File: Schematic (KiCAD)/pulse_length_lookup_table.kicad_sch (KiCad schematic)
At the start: 122 parts

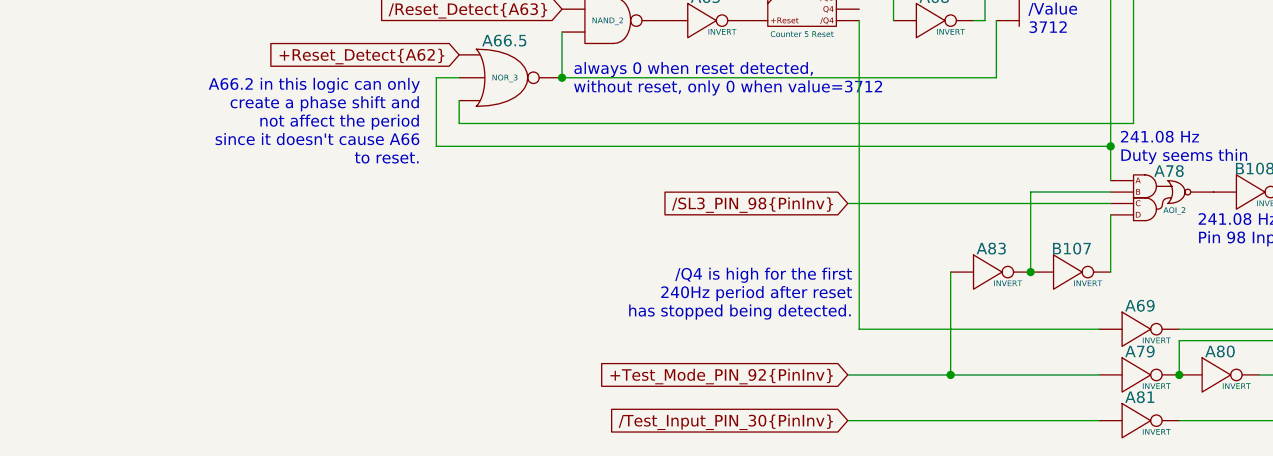
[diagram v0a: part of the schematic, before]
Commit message: Schematic and SVG Updates
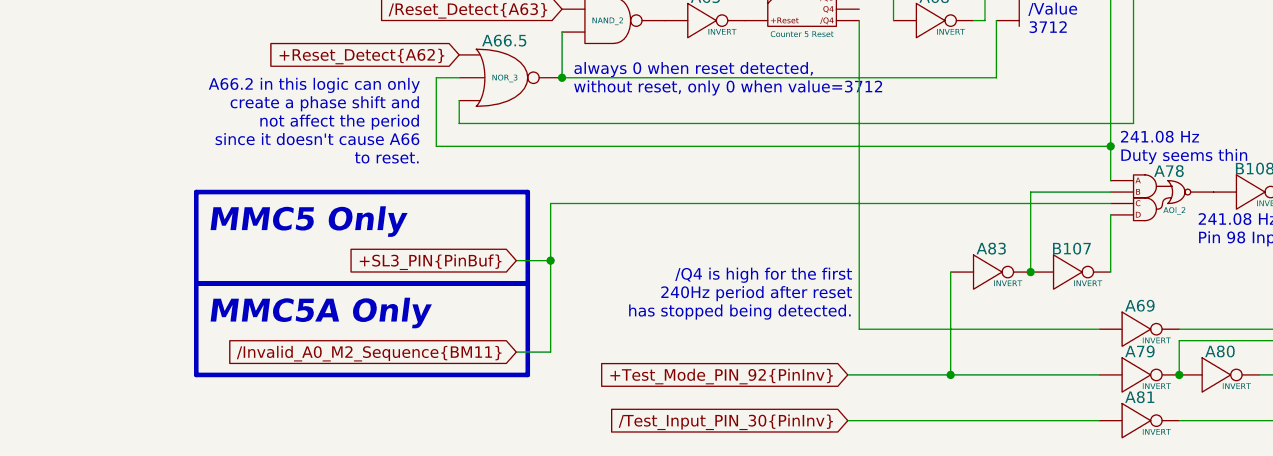
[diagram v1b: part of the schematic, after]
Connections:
- net /SL3_PIN_98{PinInv} is gone; now on net +SL3_PIN{PinBuf}: A78. (X)
- net at B108. (X): now also A78. (X); no longer A70. (X)
- net at A71. (X): now also A72. (X), A73. (X); no longer A70. (X)
- net at C16. (X): now also D47. (X); no longer C15. (X)
- net at D45. (X): now also D46. (X); no longer C16. (X)
- net at D47. (X): now also D48. (X); no longer C16. (X)
- net at D72. (X): now also C22. (X); no longer D71. (X)
- net at D92. (X): now also C26. (X); no longer D91. (X)
- net at C26. (X): now also C25. (X); no longer D92. (X)
- net at C18. (X): now also D51. (X); no longer C17. (X)
- net at D106. (X): now also C28. (X); no longer D105. (X)
- net at A58. (X): now also A57. (X), A66. (/Q7); no longer A59. (X)
- net at D66. (X): now also D65. (X); no longer C20. (X)
- net at A67. (/Q4): now also A65. (X)
- net at A66.7. (X): now also A66.4. (X); no longer A67. (/Q4)
- net at A68. (X): now also A66.4. (X); no longer A67. (/Q4)
- net at A66.6. (X): now also A66.4. (X); no longer A67. (/Q4)
- net at A69. (X): now also A77. (X); no longer A67. (/Q4)
- net at A65. (X): now also A64. (X); no longer A67. (/Q4)
- net at A66.4. (X): now also A66.5. (X), A78. (X); no longer A66.7. (X)
- net at D64. (X): now also C20. (X); no longer D63. (X)
- net at D76. (X): now also C22. (X); no longer D75. (X)
- net at D53. (X): now also C18. (X); no longer D54. (X)
- net at D96. (X): now also D95. (X); no longer C26. (X)
- net at A73. (X): now also A74. (X); no longer A82. (X)
- net at A74. (X): now also A75. (X); no longer A73. (X)
- net at D49. (X): now also C18. (X); no longer D50. (X)
- net at D55. (X): now also C18. (X); no longer D56. (X)
- net at D74. (X): now also D73. (X); no longer C22. (X)
- net at D70. (X): now also D69. (X); no longer C22. (X)
- net at D68. (X): now also D67. (X); no longer C22. (X)
- net at A77. (X): now also A82. (X); no longer A81. (X)
- net at A77. (X), A80. (X): now also A79. (X)
- net at D104. (X): now also C28. (X); no longer D103. (X)
- net at C28. (X): now also C27. (X); no longer D104. (X)
- net at D58. (X): now also C20. (X); no longer D57. (X)
- net at C20. (X): now also D62. (X); no longer D58. (X)
- net at A66.3. (X): now also A66. (/Q7); no longer A66.4. (X)
- net at D78. (X): now also C24. (X); no longer D77. (X)
- net at C24. (X): now also D88. (X); no longer D78. (X)
- net at D102. (X): now also C28. (X); no longer D101. (X)
- net at D51. (X): now also D52. (X); no longer C18. (X)
- net at D100. (X): now also C26. (X); no longer D99. (X)
- net at D60. (X): now also C20. (X); no longer D59. (X)
- net at D84. (X): now also D83. (X); no longer C24. (X)
- net at D86. (X): now also C24. (X); no longer D85. (X)
- net +SL3_PIN{PinBuf}: now reaches A78. (X)
- net +SL3_PIN{PinBuf}: no longer B108. (X)
- net at D82. (X): now also D81. (X); no longer C24. (X)
- net at D80. (X): now also D79. (X); no longer C24. (X)
- net at D90. (X): now also C26. (X); no longer D89. (X)
- net at A60. (X): now also A56. (X); no longer A61. (X)
- net at D94. (X): now also C26. (X); no longer D93. (X)
- net at A66.2. (X): now also A66.5. (X); no longer A66. (/Q7)
- net at D98. (X): now also D97. (X); no longer C26. (X)
- new net: A70. (X), B108. (X)
- new net: A70. (X), A71. (X)
- new net: C15. (X), C16. (X)
- new net: C16. (X), D45. (X)
- new net: D71. (X), D72. (X)
- new net: D91. (X), D92. (X)
- new net: C17. (X), C18. (X)
- new net: D105. (X), D106. (X)
- new net: A58. (X), A59. (X)
- new net: C20. (X), D66. (X)
- new net: A66.7. (X), A67. (/Q4)
- new net: A67. (/Q4), A68. (X)
- new net: A66.6. (X), A67. (/Q4)
- new net: A67. (/Q4), A69. (X)
- new net: A66. (/Q7), A67. (/Q4)
- new net: D63. (X), D64. (X)
- new net: D75. (X), D76. (X)
- new net: D53. (X), D54. (X)
- new net: C26. (X), D96. (X)
- new net: A73. (X), A82. (X)
- new net: D49. (X), D50. (X)
- new net: A64. (X), A66.4. (X), A66.5. (X)
- new net: D55. (X), D56. (X)
- new net: C21. (X), C22. (X)
- new net: C22. (X), D74. (X)
- new net: C22. (X), D70. (X)
- new net: C22. (X), D68. (X)
- new net: A77. (X), A81. (X)
- new net: A77. (X), A80. (X)
- new net: D103. (X), D104. (X)
- new net: D57. (X), D58. (X)
- new net: D61. (X), D62. (X)
- new net: A66.3. (X), A66.4. (X)
- new net: D77. (X), D78. (X)
- new net: C23. (X), C24. (X)
- new net: C19. (X), C20. (X)
- new net: A55. (/Q), A56. (X), A57. (X)
- new net: B43. (X), B44. (X)
- new net: B42. (X), B43. (X)
- new net: D101. (X), D102. (X)
- new net: C10. (X), D38. (Ripple_Out)
- new net: C10. (X), C9. (X)
- new net: D100. (X), D99. (X)
- new net: D59. (X), D60. (X)
- new net: D38. (Ripple_Out), D39. (Ripple_Out)
- new net: C24. (X), D84. (X)
- new net: D85. (X), D86. (X)
- new net: C11. (Ripple_Out), C12. (Ripple_Out)
- new net: B42. (X), C11. (Ripple_Out)
- new net: D87. (X), D88. (X)
- new net: C24. (X), D82. (X)
- new net: C24. (X), D80. (X)
- new net: D89. (X), D90. (X)
- new net: C8. (X), C9. (X)
- new net: A60. (X), A61. (X)
- new net: D93. (X), D94. (X)
- new net: A66. (/Q7), A66.2. (X)
- new net: A78. (X), A83. (X), B107. (X)
- new net: C26. (X), D98. (X)
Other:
- note added: "MMC5 Only"
- note added: "MMC5A Only"
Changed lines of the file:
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@@
 	(generator_version "9.0")
 	(paper "USLedger")
+	(rectangle
+		(start 186.69 222.25)
+		(end 223.52 232.41)
+		(stroke
+			(width 0.508)
+			(type default)
+		)
+		(fill
+			(type none)
+		)
+	)
+	(rectangle
+		(start 186.69 212.09)
+		(end 223.52 222.25)
+		(stroke
+			(width 0.508)
+			(type default)
+		)
+		(fill
+			(type none)
+		)
+	)
 	(text "always 0 when reset detected,\nwithout reset, only 0 when value=3712"
 		(exclude_from_sim no)
@@
 		)
 	)
-	(text "The reset inputs of ALL these\ncounters seem to be /Reset.\nHard to see why this acts different\nthan T-FF counters elsewhere."
+	(text "MMC5 Only"
 		(exclude_from_sim no)
-		(at 220.726 168.148 0)
-		(effects
-			(font
-				(size 1.27 1.27)
-			)
-		)
-	)
-	(text "894.886 kHz"
-		(exclude_from_sim no)
-		(at 337.82 147.574 0)
-		(effects
-			(font
-				(size 1.27 1.27)
-			)
-			(justify right)
-		)
-	)
-	(text "0=Reset Held By A67.Q4 or Pin 30"
-		(exclude_from_sim no)
-		(at 329.946 228.6 0)
-		(effects
-			(font
-				(size 1.27 1.27)
-			)
-			(justify left)
-		)
-	)
-	(text "/Value\n3712"
-		(exclude_from_sim no)
-		(at 279.146 193.04 0)
-		(effects
-			(font
-				(size 1.27 1.27)
-			)
-			(justify left)
-		)
-	)
-	(text "These counters count \"down\"\nthe preloaded period value.\n\nThis means either the outputs\nor preload inputs are inverted."
-		(exclude_from_sim no)
-		(at 292.862 33.528 0)
-		(effects
-			(font
-				(size 1.27 1.27)
-			)
-			(justify left)
-		)
-	)
-	(text "Important:\nA63 resets\nQ4 of A67."
-		(exclude_from_sim no)
-		(at 246.634 186.69 0)
-		(effects
-			(font
-				(size 1.27 1.27)
-			)
-			(justify right)
-		)
-	)
-	(text "5-Bit to 7-Bit\nPulse Length Lookup Table"
-		(exclude_from_sim no)
-		(at 81.534 20.32 0)
+		(at 187.96 215.392 0)
 		(effects
 			(font
@@
 				(italic yes)
 			)
-		)
-	)
-	(text "447.443 kHz\n50% duty"
+			(justify left)
+		)
+	)
+	(text "The reset inputs of ALL these\ncounters seem to be /Reset.\nHard to see why this acts different\nthan T-FF counters elsewhere."
 		(exclude_from_sim no)
-		(at 268.732 159.004 0)
+		(at 220.726 168.148 0)
+		(effects
+			(font
+				(size 1.27 1.27)
+			)
+		)
+	)
+	(text "894.886 kHz"
+		(exclude_from_sim no)
+		(at 337.82 147.574 0)
+		(effects
+			(font
+				(size 1.27 1.27)
+			)
+			(justify right)
+		)
+	)
+	(text "0=Reset Held By A67.Q4 or Pin 30"
+		(exclude_from_sim no)
+		(at 329.946 228.6 0)
 		(effects
 			(font
@@
 		)
 	)
-	(text "/Q4 is high for the first\n240Hz period after reset\nhas stopped being detected."
+	(text "/Value\n3712"
 		(exclude_from_sim no)
-		(at 259.588 223.52 0)
-		(effects
-			(font
-				(size 1.27 1.27)
-			)
-			(justify right)
-		)
-	)
-	(text "$5007 Register\nPulse 2 Length Counter"
+		(at 279.146 193.04 0)
+		(effects
+			(font
+				(size 1.27 1.27)
+			)
+			(justify left)
+		)
+	)
+	(text "These counters count \"down\"\nthe preloaded period value.\n\nThis means either the outputs\nor preload inputs are inverted."
 		(exclude_from_sim no)
-		(at 279.908 70.612 0)
+		(at 292.862 33.528 0)
+		(effects
+			(font
+				(size 1.27 1.27)
+			)
+			(justify left)
+		)
+	)
+	(text "Important:\nA63 resets\nQ4 of A67."
+		(exclude_from_sim no)
+		(at 246.634 186.69 0)
+		(effects
+			(font
+				(size 1.27 1.27)
+			)
+			(justify right)
+		)
+	)
+	(text "5-Bit to 7-Bit\nPulse Length Lookup Table"
+		(exclude_from_sim no)
+		(at 81.534 20.32 0)
 		(effects
 			(font
@@
 		)
 	)
+	(text "447.443 kHz\n50% duty"
+		(exclude_from_sim no)
+		(at 268.732 159.004 0)
+		(effects
+			(font
+				(size 1.27 1.27)
+			)
+			(justify left)
+		)
+	)
+	(text "/Q4 is high for the first\n240Hz period after reset\nhas stopped being detected."
+		(exclude_from_sim no)
+		(at 259.588 223.52 0)
+		(effects
+			(font
+				(size 1.27 1.27)
+			)
+			(justify right)
+		)
+	)
+	(text "$5007 Register\nPulse 2 Length Counter"
+		(exclude_from_sim no)
+		(at 279.908 70.612 0)
+		(effects
+			(font
+				(size 2.54 2.54)
+				(thickness 0.508)
+				(bold yes)
+				(italic yes)
+			)
+		)
+	)
 	(text "All of these outputs are\n241.08 Hz\n-or- \nPin 98 Input"
 		(exclude_from_sim no)
@@
 		)
 	)
+	(text "MMC5A Only"
+		(exclude_from_sim no)
+		(at 187.96 225.552 0)
+		(effects
+			(font
+				(size 2.54 2.54)
+				(thickness 0.508)
+				(bold yes)
+				(italic yes)
+			)
+			(justify left)
+		)
+	)
 	(text "241.08 Hz or\nPin 98 Input"
 		(exclude_from_sim no)
@@
 			)
 		)
+	)
+	(junction
+		(at 226.06 219.71)
+		(diameter 0)
+		(color 0 0 0 0)
 	)
 	(junction
@@
 	(wire
 		(pts
+			(xy 226.06 213.36) (xy 226.06 219.71)
+		)
+		(stroke
+			(width 0)
+			(type default)
+		)
+	)
+	(wire
+		(pts
 			(xy 247.65 151.13) (xy 247.65 171.45)
 		)
@@
 	(wire
 		(pts
+			(xy 226.06 213.36) (xy 288.29 213.36)
+		)
+		(stroke
+			(width 0)
+			(type default)
+		)
+	)
+	(wire
+		(pts
 			(xy 215.9 204.47) (xy 215.9 201.93)
 		)
@@
 	(wire
 		(pts
+			(xy 226.06 229.87) (xy 222.25 229.87)
+		)
+		(stroke
+			(width 0)
+			(type default)
+		)
+	)
+	(wire
+		(pts
 			(xy 220.98 160.02) (xy 220.98 149.86)
 		)
@@
 	(wire
 		(pts
-			(xy 259.08 213.36) (xy 288.29 213.36)
-		)
-		(stroke
-			(width 0)
-			(type default)
-		)
-	)
-	(wire
-		(pts
 			(xy 146.05 152.4) (xy 146.05 129.54)
 		)
@@
 	(wire
 		(pts
+			(xy 226.06 219.71) (xy 226.06 229.87)
+		)
+		(stroke
+			(width 0)
+			(type default)
+		)
+	)
+	(wire
+		(pts
 			(xy 260.35 187.96) (xy 264.16 187.96)
 		)
@@
 		(pts
 			(xy 267.97 97.79) (xy 273.05 97.79)
+		)
+		(stroke
+			(width 0)
+			(type default)
+		)
+	)
+	(wire
+		(pts
+			(xy 222.25 219.71) (xy 226.06 219.71)
 		)
 		(stroke
@@
 		)
 	)
+	(global_label "+SL3_PIN{PinBuf}"
+		(shape input)
+		(at 222.25 219.71 180)
+		(fields_autoplaced yes)
+		(effects
+			(font
+				(size 1.27 1.27)
+			)
+			(justify right)
+		)
+		(property "Intersheetrefs" "${INTERSHEET_REFS}"
+			(at 202.2105 219.71 0)
+			(effects
+				(font
+					(size 1.27 1.27)
+				)
+				(justify right)
+				(hide yes)
+			)
+		)
+	)
 	(global_label "1"
 		(shape input)
@@
 		)
 	)
-	(global_label "{slash}SL3_PIN_98{PinInv}"
-		(shape input)
-		(at 259.08 213.36 180)
-		(fields_autoplaced yes)
-		(effects
-			(font
-				(size 1.27 1.27)
-			)
-			(justify right)
-		)
-		(property "Intersheetrefs" "${INTERSHEET_REFS}"
-			(at 281.8409 213.36 0)
-			(effects
-				(font
-					(size 1.27 1.27)
-				)
-				(justify left)
-				(hide yes)
-			)
+	(global_label "{slash}Invalid_A0_M2_Sequence{BM11}"
+		(shape input)
+		(at 222.25 229.87 180)
+		(fields_autoplaced yes)
+		(effects
+			(font
+				(size 1.27 1.27)
+			)
+			(justify right)
+		)
+		(property "Intersheetrefs" "${INTERSHEET_REFS}"
+			(at 187.9384 229.87 0)
+			(effects
+				(font
+					(size 1.27 1.27)
+				)
+				(justify right)
+				(hide yes)
+			)
